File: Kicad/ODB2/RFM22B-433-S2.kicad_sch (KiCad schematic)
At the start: 0 parts

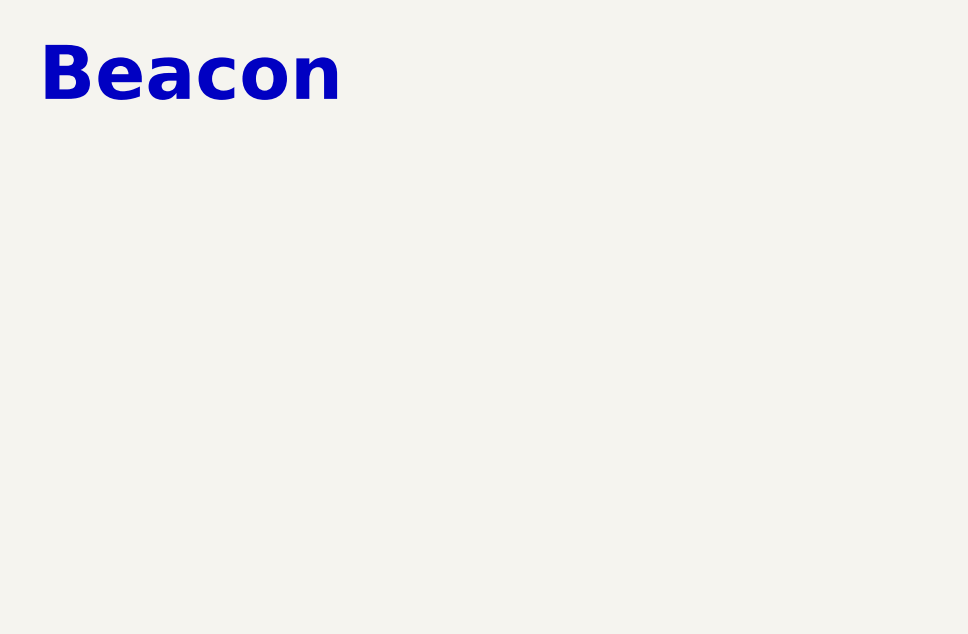
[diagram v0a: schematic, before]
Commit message: add rfm
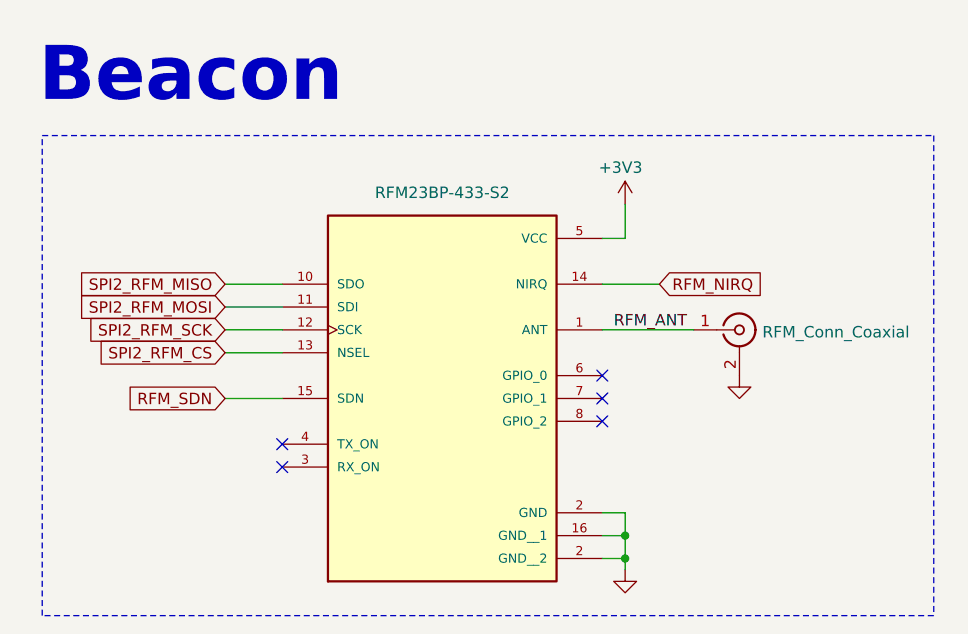
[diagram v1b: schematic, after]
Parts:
- added J6: RFM_Conn_Coaxial, symbol Connector:Conn_Coaxial
- added U9: RFM23BP-433-S2, RFM23BP-433-S2:MODULE_RFM23BP-433-S2, symbol ODB2:RFM23BP-433-S2
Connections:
- new net +3V3: U9.5 (VCC)
- new net GND: J6.2 (Ext), U9.16 (GND__1), U9.2 (GND__2)
- new net RFM_ANT: J6.1 (In), U9.1 (ANT)
- new net RFM_NIRQ: U9.14 (NIRQ)
- new net RFM_SDN: U9.15 (SDN)
- new net SPI2_RFM_CS: U9.13 (NSEL)
- new net SPI2_RFM_MISO: U9.10 (SDO)
- new net SPI2_RFM_MOSI: U9.11 (SDI)
- new net SPI2_RFM_SCK: U9.12 (SCK)
- no-connect marks 0 -> 5
